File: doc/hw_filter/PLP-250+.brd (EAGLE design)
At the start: 27.9 x 30 mm, 3 parts

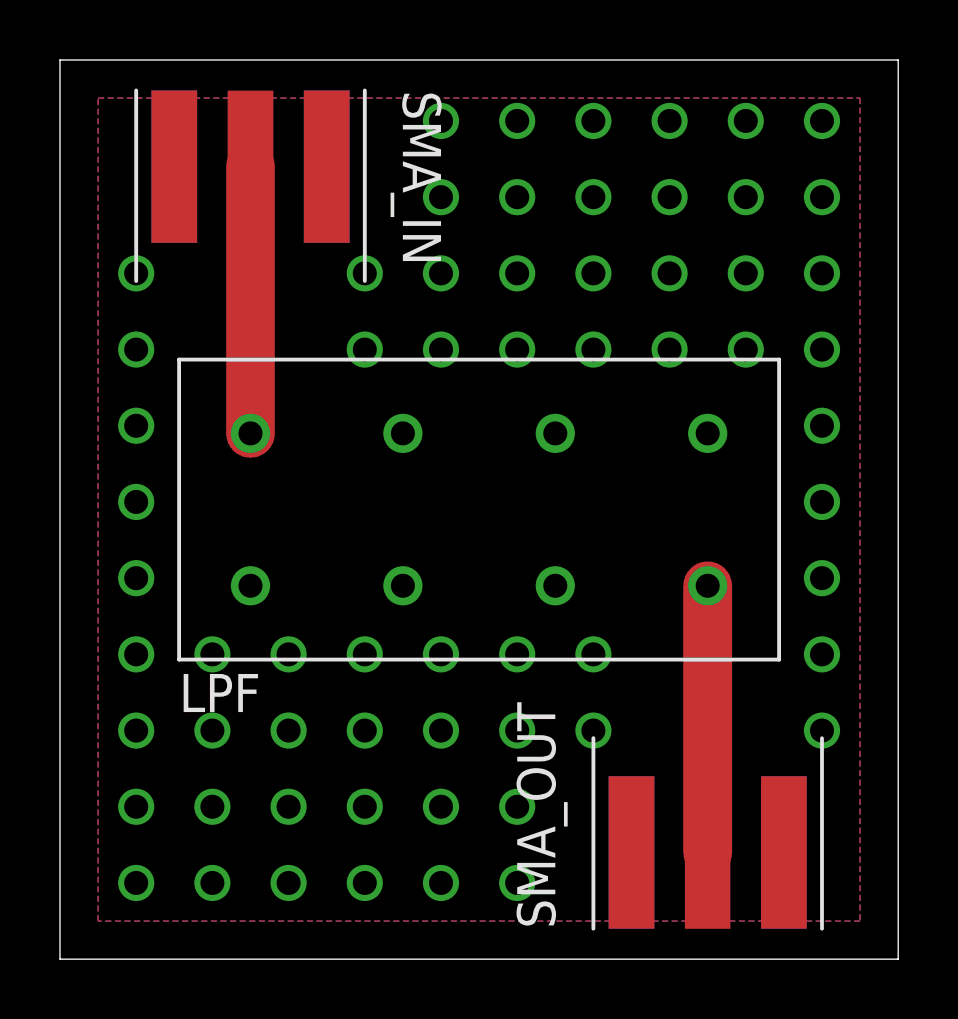
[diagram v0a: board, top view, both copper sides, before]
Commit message: updated libraries
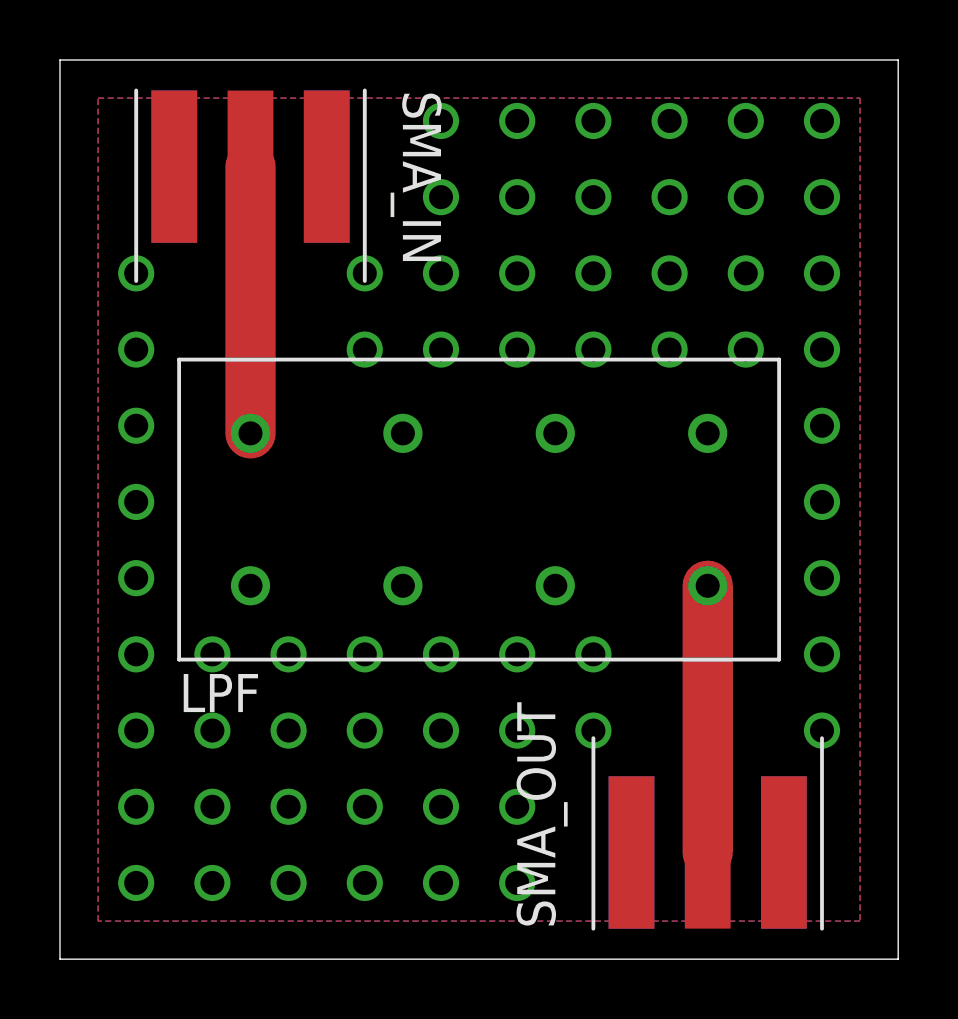
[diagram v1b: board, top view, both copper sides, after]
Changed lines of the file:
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@@
 <contactref element="SMA_IN" pad="SIG"/>
 <contactref element="LPF" pad="P1"/>
-<wire x1="6.35" y1="26.416" x2="6.35" y2="17.526" width="1.6256" layer="1"/>
+<wire x1="6.35" y1="26.416" x2="6.35" y2="17.526" width="1.6764" layer="1"/>
 </signal>
 <signal name="N$2">
 <contactref element="LPF" pad="P8"/>
 <contactref element="SMA_OUT" pad="SIG"/>
-<wire x1="21.59" y1="3.556" x2="21.59" y2="12.446" width="1.6256" layer="1"/>
+<wire x1="21.59" y1="3.556" x2="21.59" y2="12.446" width="1.6764" layer="1"/>
 </signal>
 <signal name="GND">
-<polygon width="0.4064" layer="1">
+<polygon width="0.4064" layer="1" isolate="0.254">
 <vertex x="1.27" y="28.702"/>
 <vertex x="26.67" y="28.702"/>
@@
 <vertex x="1.27" y="1.27"/>
 </polygon>
-<polygon width="0.4064" layer="16">
+<polygon width="0.4064" layer="16" isolate="0.254">
 <vertex x="1.27" y="28.702"/>
 <vertex x="26.67" y="28.702"/>
